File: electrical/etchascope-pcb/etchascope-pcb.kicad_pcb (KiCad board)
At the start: 2 copper layers, 50 x 116 mm, 18 parts, among them SW1 RotaryEncoder_Switch, U3 ADXL343

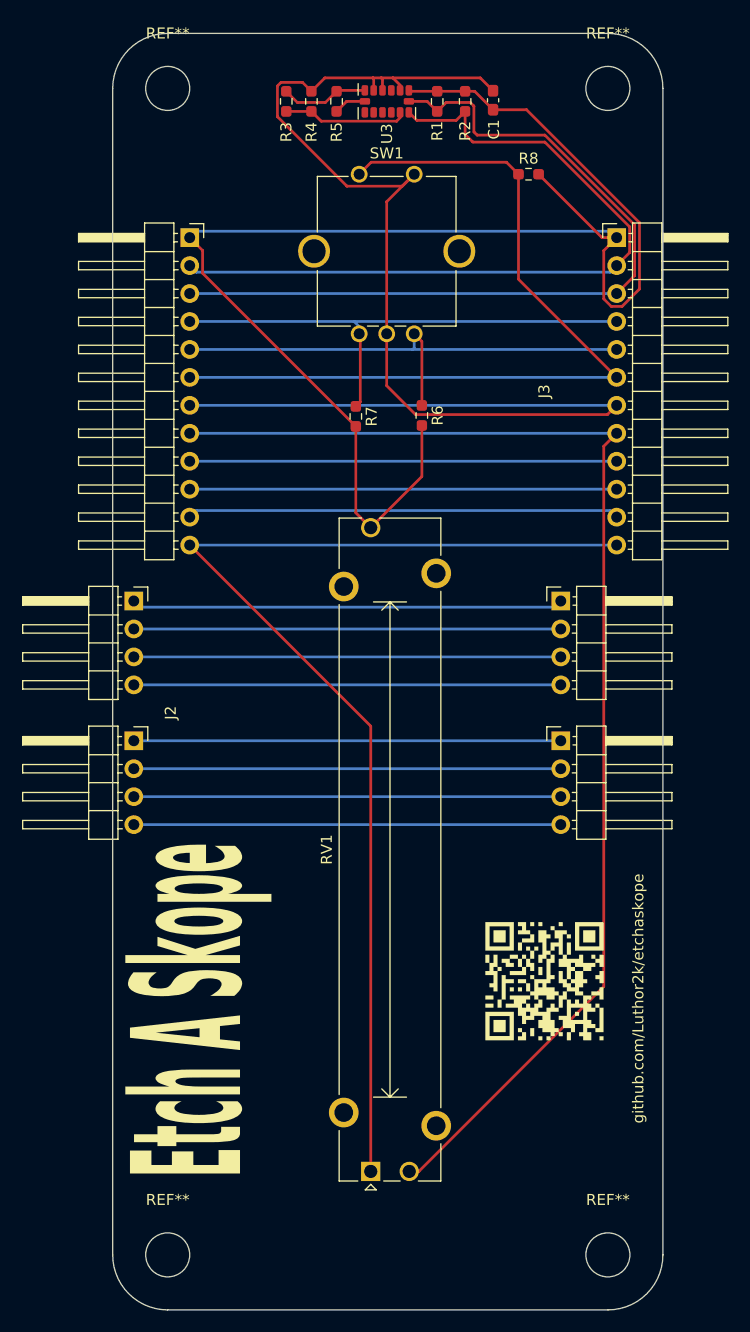
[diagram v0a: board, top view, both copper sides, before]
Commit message: logo added
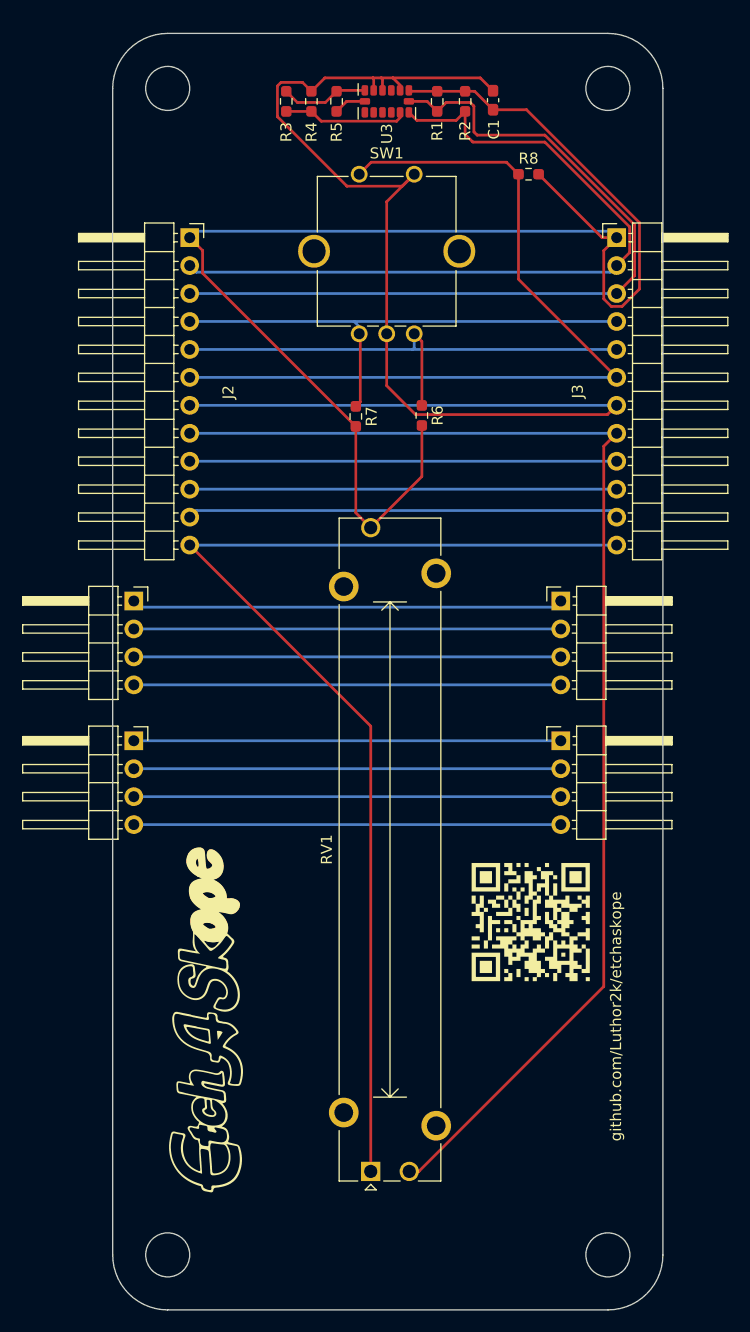
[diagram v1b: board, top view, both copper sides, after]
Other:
- board text removed: "Etch A Skope"

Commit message: tidied up connectors and logo
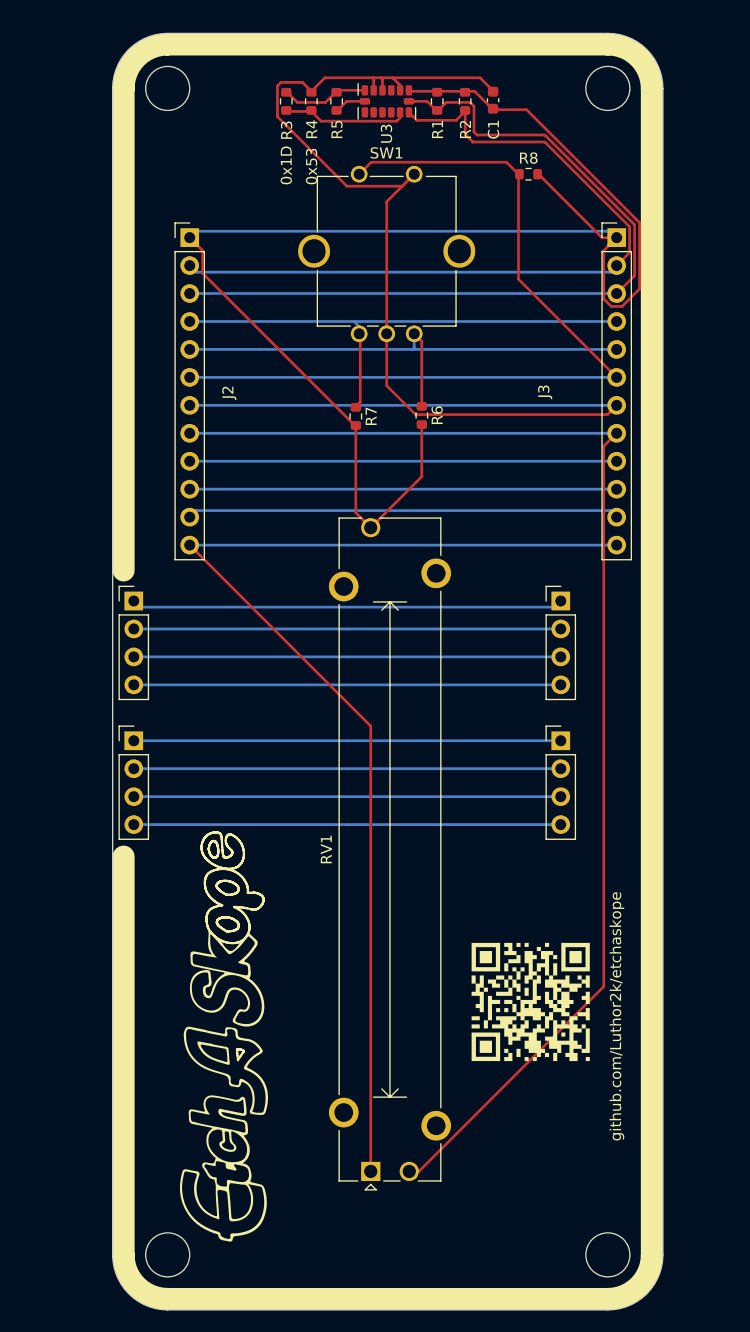
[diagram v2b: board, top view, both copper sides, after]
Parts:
- C1: footprint Capacitor_SMD:C_0603_1608Metric_Pad1.08x0.95mm_HandSolder -> Capacitor_SMD:C_0603_1608Metric
- R1, R2, R3, R4, R5, R6, R7, R8: footprint Resistor_SMD:R_0603_1608Metric_Pad0.98x0.95mm_HandSolder -> Resistor_SMD:R_0603_1608Metric
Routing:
- net VSS: track 143.4 -> 221.5 mm
- net /GP26: track 46.8 -> 124.4 mm
- net /SDA: track 69.6 -> 147.2 mm
- net /SCL: track 72.9 -> 150.5 mm
- net /SCOPE3V3: track 39.3 -> 0.00 mm
- net /SIGNAL_Y: track 38.8 -> 0.00 mm
- net /SIGNAL_X: track 38.8 -> 0.00 mm
- net /SIGNAL_GND: track 38.8 -> 0.00 mm
- net /SIGNAL3V3: track 38.8 -> 0.00 mm
- net /SCOPE_Y: track 38.8 -> 0.00 mm
- net /SCOPE_X: track 38.8 -> 0.00 mm
- net /SCOPE_GND: track 38.8 -> 0.00 mm
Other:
- board text added: "0x1D"
- board text added: "0x53"
